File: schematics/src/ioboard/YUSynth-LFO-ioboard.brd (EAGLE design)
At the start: 160 x 100 mm, 1 part, among them IC1 TL074P

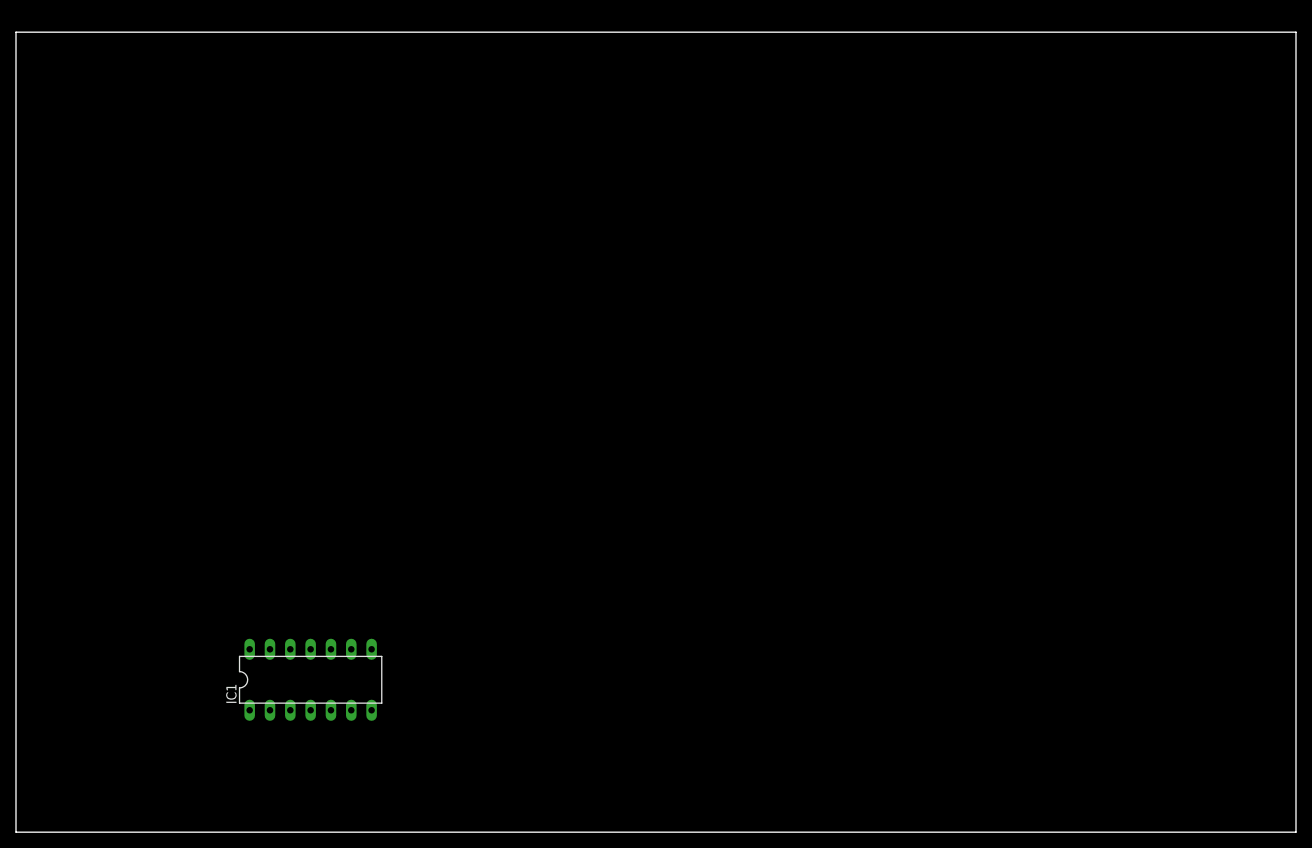
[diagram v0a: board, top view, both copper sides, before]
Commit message: initial designs
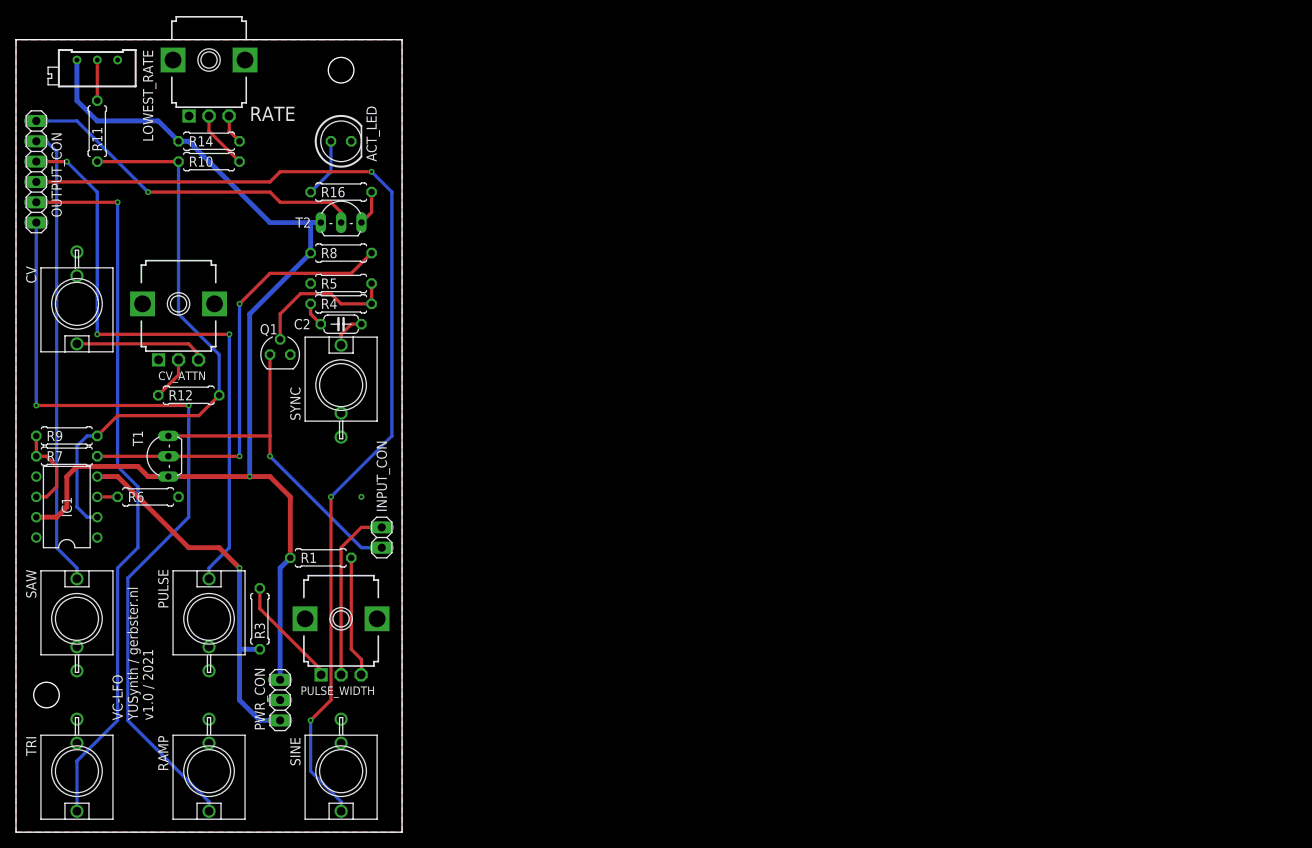
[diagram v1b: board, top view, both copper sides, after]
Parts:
- added ACT_LED: (no value), led:LED5MM
- added C2: 10nF, rcl:C050-024X044
- added CV, PULSE, RAMP, SAW, SINE, SYNC, TRI: (no value), thonkiconn:WQP-PJ301M-12_JACK
- added CV_ATTN: 50k lin, TomW:EVUF
- added INPUT_CON: (no value), pinhead:1X02
- added LOWEST_RATE: 50k, rcl:RTRIM64X
- added OUTPUT_CON: (no value), pinhead:1X06
- added PULSE_WIDTH, RATE: 10k lin, TomW:EVUF
- added PWR_CON: (no value), pinhead:1X03
- added Q1: BS170, transistor-small-signal:SOT54E
- added R1, R3: 15k, rcl:0207/7
- added R10, R11, R12, R5, R9: 100k, rcl:0207/7
- added R14: 12k, rcl:0207/7
- added R16: 1k, rcl:0207/7
- added R4: 10k, rcl:0207/7
- added R6: 8.2k, rcl:0207/7
- added R7: 27k, rcl:0207/7
- added R8: 820R, rcl:0207/7
- added T1: (no value), transistor:TO92-EBC
- added T2: (no value), transistor:TO92-CBE
- IC1: value TL074P -> LM741P; device linear:DIL14 -> linear:DIL08
- moved IC1 37.4 mm to (6.35, 40.6), turned to 90 degrees
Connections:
- removed net V+: IC1.4
- removed net V-: IC1.11
- new net +12V: IC1.7, LOWEST_RATE.3, PWR_CON.1, R1.2, R14.1, R8.1, T1.E, T2.C
- new net -12V: IC1.4, PWR_CON.3, R3.1
- new net CV: INPUT_CON.1, Q1.D, T1.C
- new net GND: ACT_LED.K, CV.P$3, CV_ATTN.1, LOWEST_RATE.1, PULSE.P$3, PWR_CON.2, Q1.S, R5.2, R6.2, RAMP.P$3, RATE.1, SAW.P$3, SINE.P$3, SYNC.P$3, TRI.P$3
- new net LED: OUTPUT_CON.6, T2.B
- new net N$1: PULSE_WIDTH.1, R3.2
- new net N$10: R14.2, RATE.3
- new net N$11: R10.2, RATE.2
- new net N$13: IC1.2, R10.1, R11.1, R12.1, R9.2
- new net N$14: LOWEST_RATE.2, R11.2
- new net N$15: CV_ATTN.2, R12.2
- new net N$16: CV.P$1, CV_ATTN.3
- new net N$17: R16.1, T2.E
- new net N$18: ACT_LED.A, R16.2
- new net N$2: PULSE_WIDTH.3, R1.1
- new net N$3: C2.1, SYNC.P$1
- new net N$4: C2.2, R4.2
- new net N$5: Q1.G, R4.1, R5.1
- new net N$7: IC1.3, R6.1
- new net N$8: IC1.6, R7.2, R9.1
- new net N$9: R7.1, R8.2, T1.B
- new net PULSE_OUT: OUTPUT_CON.4, PULSE.P$1
- new net PULSE_WIDTH: INPUT_CON.2, PULSE_WIDTH.2
- new net RAMP_OUT: OUTPUT_CON.1, RAMP.P$1
- new net SAW_OUT: OUTPUT_CON.5, SAW.P$1
- new net SINE_OUT: OUTPUT_CON.3, SINE.P$1
- new net TRI_OUT: OUTPUT_CON.2, TRI.P$1
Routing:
- net +12V: track 0.00 -> 139.6 mm, vias 0 -> 1
- net SINE_OUT: track 0.00 -> 129.2 mm, vias 0 -> 3
- net RAMP_OUT: track 0.00 -> 100.0 mm, vias 0 -> 2
- net TRI_OUT: track 0.00 -> 90.5 mm, vias 0 -> 1
- net PULSE_OUT: track 0.00 -> 75.1 mm, vias 0 -> 3
- net N$13: track 0.00 -> 72.6 mm
- net SAW_OUT: track 0.00 -> 57.5 mm
- net N$9: track 0.00 -> 56.0 mm, vias 0 -> 2
- net -12V: track 0.00 -> 47.7 mm, vias 0 -> 1
- net LED: track 0.00 -> 44.1 mm, vias 0 -> 1
- net CV: track 0.00 -> 44.1 mm, vias 0 -> 1
- net PULSE_WIDTH: track 0.00 -> 22.0 mm
- net N$5: track 0.00 -> 18.7 mm
- net N$16: track 0.00 -> 16.5 mm
- net N$2: track 0.00 -> 15.2 mm
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- added copper zone on layer 1, net GND
- added copper zone on layer 16, net GND
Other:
- board size 160 x 100 mm -> 48.3 x 99.1 mm
- board text added: "VC-LFO YUSynth / gerbster.nl v1.0 / 2021"
